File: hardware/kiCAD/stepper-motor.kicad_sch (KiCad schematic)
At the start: 4 parts, among them J1 Conn_01x04, J2 Conn_01x06

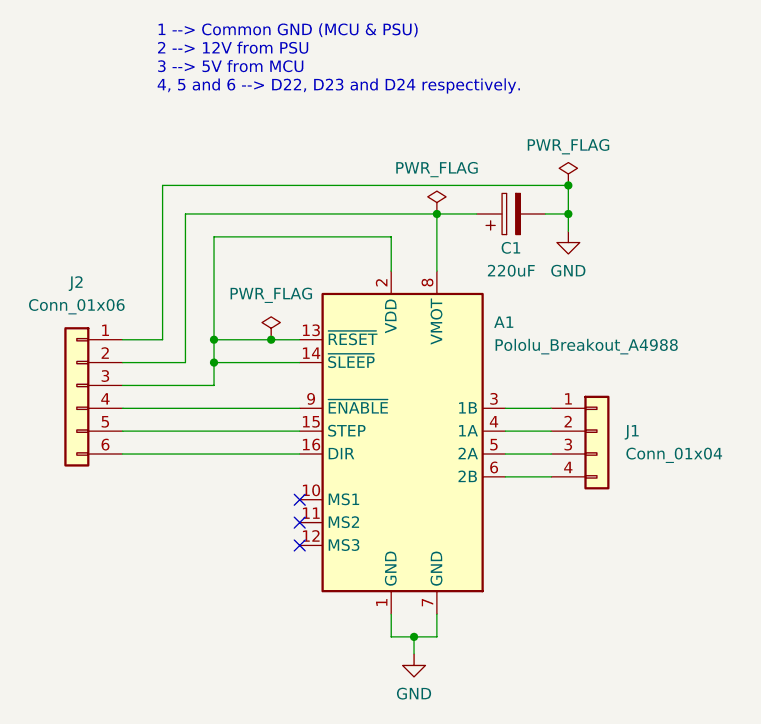
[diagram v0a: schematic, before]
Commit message: fix: changed pins
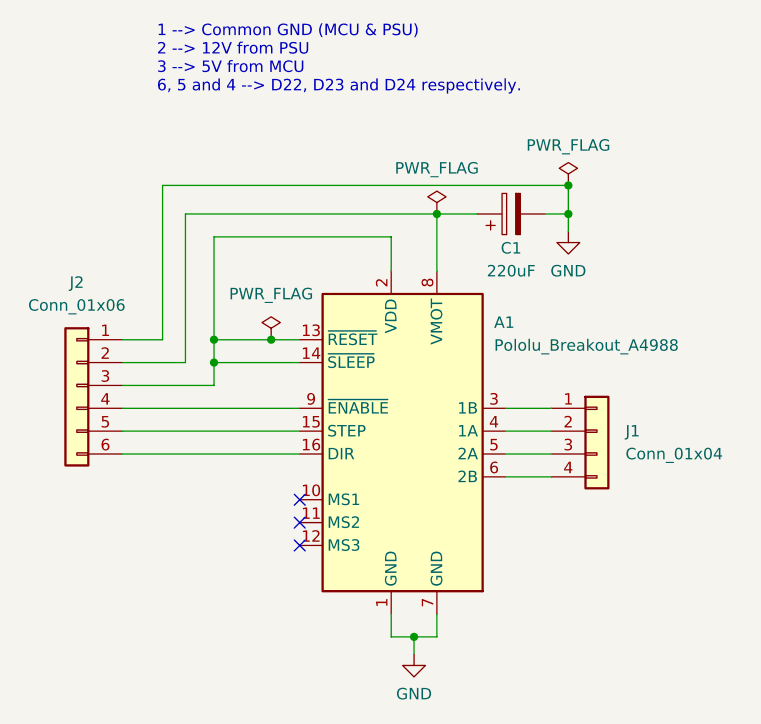
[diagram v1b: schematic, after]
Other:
- note added: "1 --> Common GND (MCU & PSU) 2 --> 12V from PSU 3 --> 5V from MCU 6, 5 and 4 --> D22, D23 and D24 respectively."
- note removed: "1 --> Common GND (MCU & PSU) 2 --> 12V from PSU 3 --> 5V from MCU 4, 5 and 6 --> D22, D23 and D24 respectively."
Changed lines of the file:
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@@
     (stroke (width 0) (type default))
   )
-  (text "1 --> Common GND (MCU & PSU)\n2 --> 12V from PSU\n3 --> 5V from MCU\n4, 5 and 6 --> D22, D23 and D24 respectively."
+  (text "1 --> Common GND (MCU & PSU)\n2 --> 12V from PSU\n3 --> 5V from MCU\n6, 5 and 4 --> D22, D23 and D24 respectively."
     (at 120.015 45.085 0)
     (effects (font (size 1.27 1.27)) (justify left bottom))
